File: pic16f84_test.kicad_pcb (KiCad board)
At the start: 2 copper layers, 59.9 x 20.6 mm, 20 parts, among them J1 ICSP, J2 Conn_01x03, Q1 2N7002, Q2 2N7002, Q3 2N7002, Q4 2N7002, U1 PIC16F54-IP

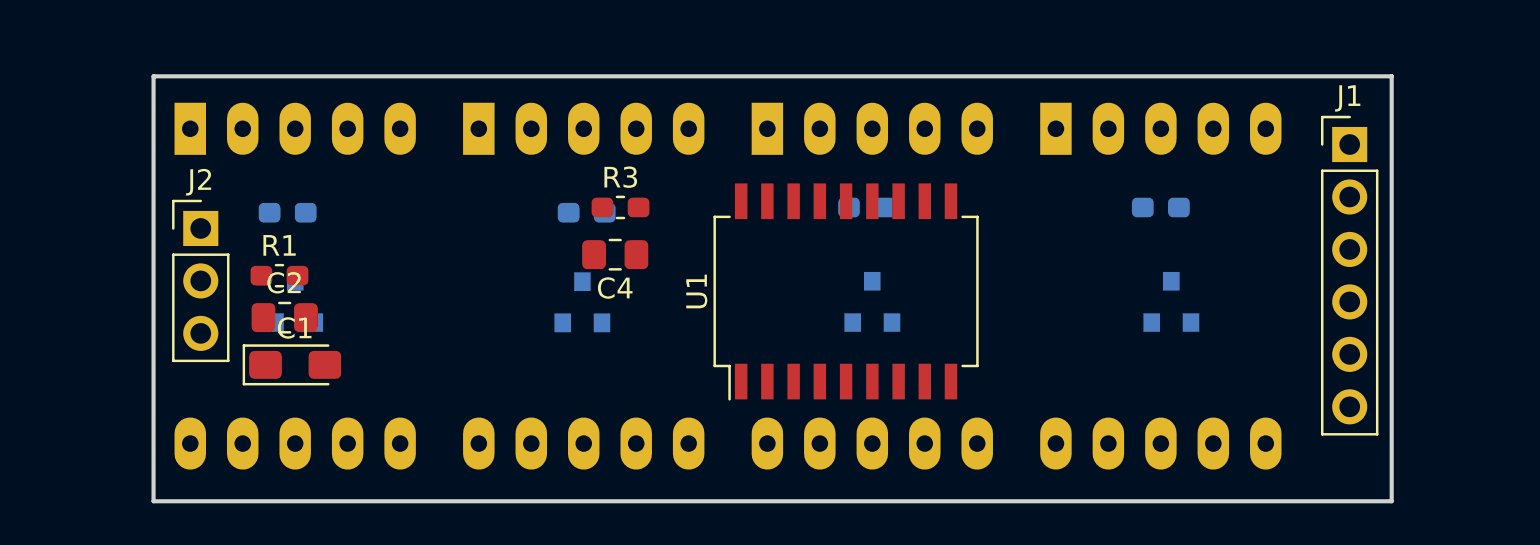
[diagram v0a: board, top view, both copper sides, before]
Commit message: done with revision 0.01
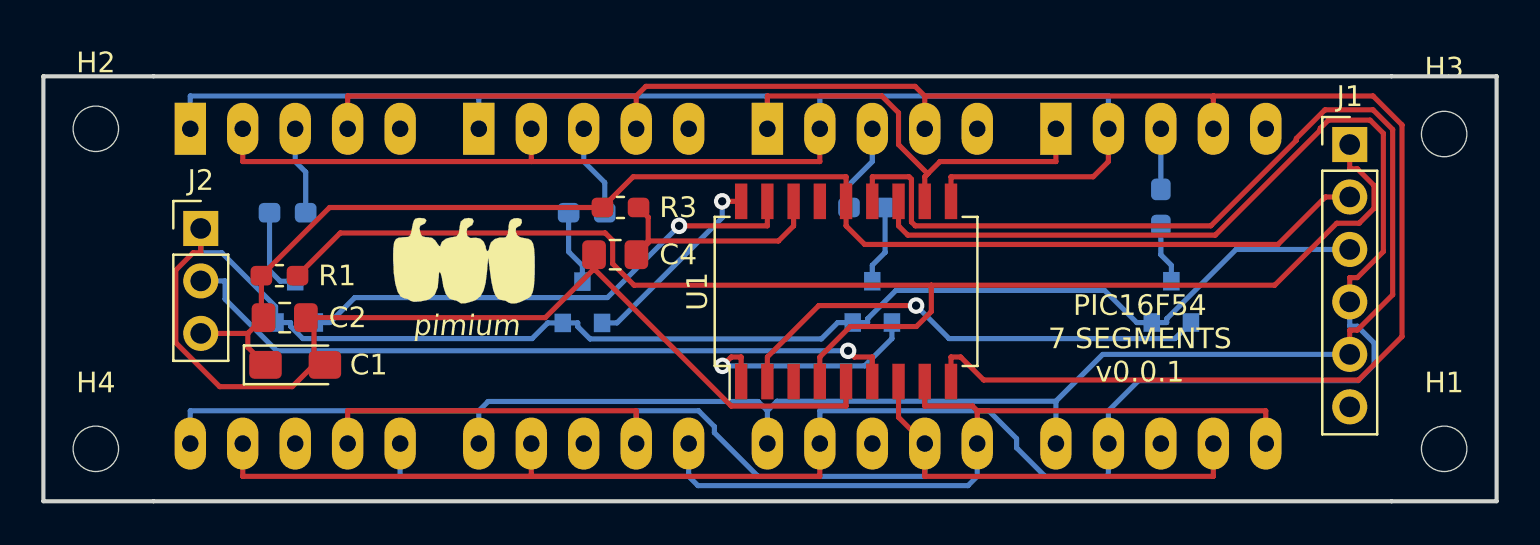
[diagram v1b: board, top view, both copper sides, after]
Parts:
- added G***: LOGO, custom_logo:pimium_paprika_7mm, F.Cu at (112.0, 97.8)
- added H1: MountingHole, MountingHole:MountingHole_2.2mm_M2, F.Cu at (159.5, 105.7)
- added H2: MountingHole, MountingHole:MountingHole_2.2mm_M2, F.Cu at (94.2, 90.2)
- added H3: MountingHole, MountingHole:MountingHole_2.2mm_M2, F.Cu at (159.5, 90.4)
- added H4: MountingHole, MountingHole:MountingHole_2.2mm_M2, F.Cu at (94.2, 105.7)
- turned R7 to 90 degrees
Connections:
- AFF1 pad 10: /SEG_G -> /PGD
- AFF1 pad 9: /SEG_F -> /PGC
- AFF2 pad 10: /SEG_G -> /PGD
- AFF2 pad 9: /SEG_F -> /PGC
- AFF3 pad 10: /SEG_G -> /PGD
- AFF3 pad 9: /SEG_F -> /PGC
- AFF4 pad 10: /SEG_G -> /PGD
- AFF4 pad 9: /SEG_F -> /PGC
- J1 pad 4: (no net) -> /PGC
- J1 pad 5: (no net) -> /PGD
- U1 pad 12: /SEG_F -> /PGC
- U1 pad 13: /SEG_G -> /PGD
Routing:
- net GND: track 0.00 -> 112.1 mm
- net /PGD: track 0.00 -> 107.8 mm
- net /PGC: track 0.00 -> 107.1 mm
- net /SEG_C: track 0.00 -> 93.0 mm
- net Net-(J1-Pad1): track 0.00 -> 68.8 mm
- net VCC: track 0.00 -> 65.7 mm
- net /SEG_D: track 0.00 -> 60.5 mm
- net /SEG_A: track 0.00 -> 56.5 mm
- net /SEG_B: track 0.00 -> 54.0 mm
- net /SEG_E: track 0.00 -> 53.9 mm
- net /DIO: track 0.00 -> 35.7 mm, vias 0 -> 1
- net /DIG_0: track 0.00 -> 25.0 mm, vias 0 -> 1
- net /DIG_3: track 0.00 -> 23.7 mm, vias 0 -> 1
- net /DIG_2: track 0.00 -> 11.8 mm, vias 0 -> 1
- net Net-(C4-Pad1): track 0.00 -> 11.2 mm
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- added copper zone on B.Cu, net GND
- added copper zone on F.Cu, net GND
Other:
- board size 59.9 x 20.6 mm -> 70.4 x 20.6 mm
- board text added: "PIC16F54 7 SEGMENTS v0.0.1"
